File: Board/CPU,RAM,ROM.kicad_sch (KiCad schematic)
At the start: 25 parts, among them IC3 74LVC125, IC6 741G04DBV, IC7 74LVC138, U1 IS61C5128AL-10TLI, X3 SG-8002CE

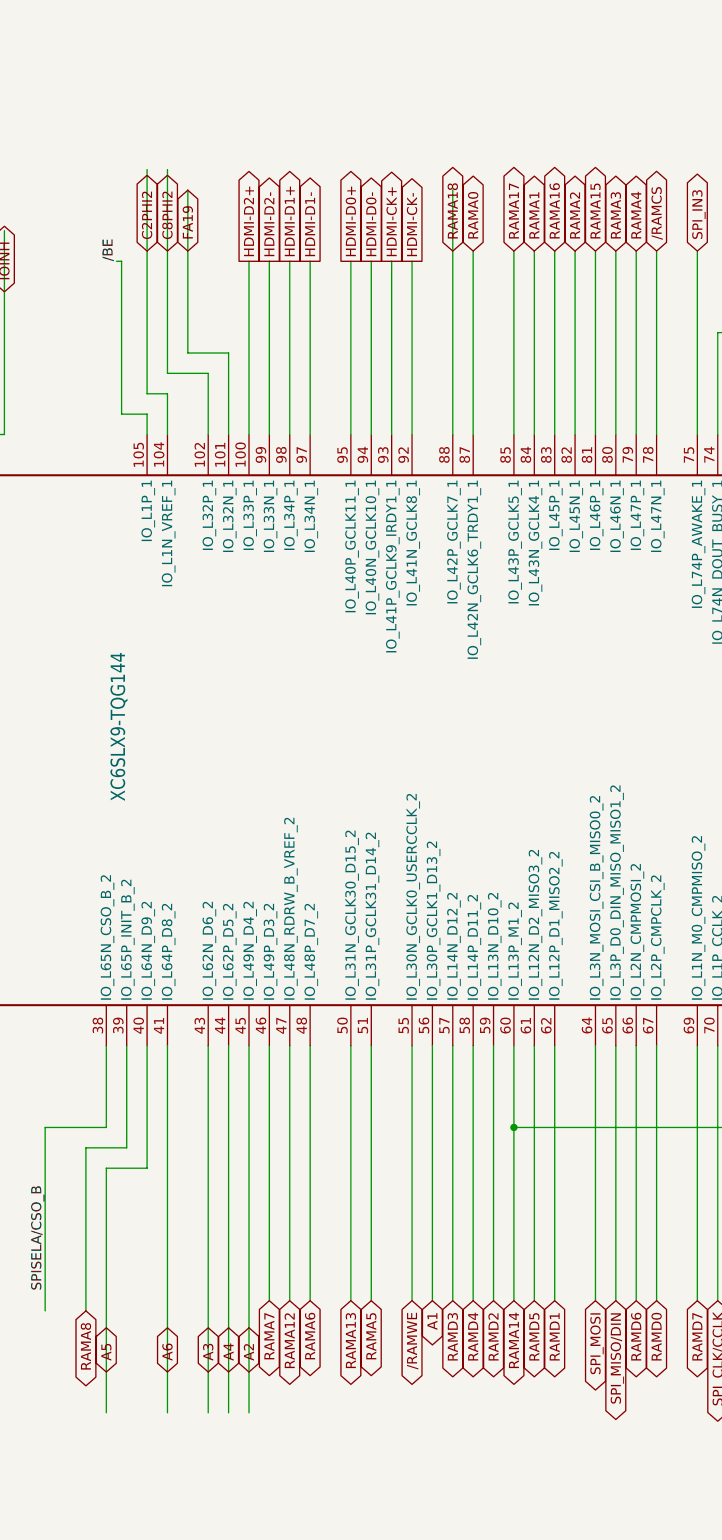
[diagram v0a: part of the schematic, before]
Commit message: update
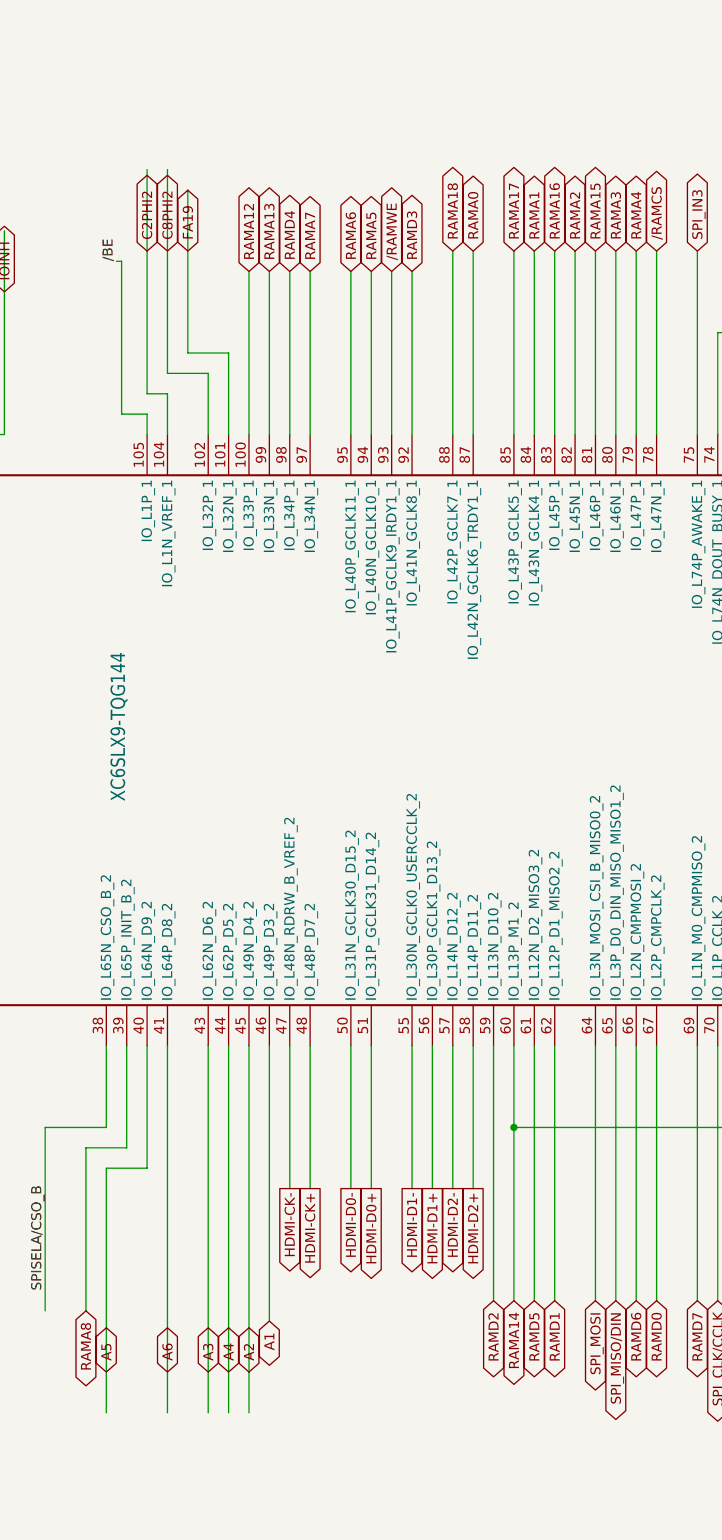
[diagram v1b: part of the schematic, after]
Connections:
- net /RAMWE: now also U$2.93 (IO_L41P_GCLK9_IRDY1_1); no longer U$2.55 (IO_L30N_GCLK0_USERCCLK_2)
- net A1: now also U$2.46 (IO_L49P_D3_2); no longer U$2.56 (IO_L30P_GCLK1_D13_2)
- net HDMI-CK+: now also U$2.48 (IO_L48P_D7_2); no longer U$2.93 (IO_L41P_GCLK9_IRDY1_1)
- net HDMI-CK-: now also U$2.47 (IO_L48N_RDRW_B_VREF_2); no longer U$2.92 (IO_L41N_GCLK8_1)
- net HDMI-D0+: now also U$2.51 (IO_L31P_GCLK31_D14_2); no longer U$2.95 (IO_L40P_GCLK11_1)
- net HDMI-D0-: now also U$2.50 (IO_L31N_GCLK30_D15_2); no longer U$2.94 (IO_L40N_GCLK10_1)
- net HDMI-D1+: now also U$2.56 (IO_L30P_GCLK1_D13_2); no longer U$2.98 (IO_L34P_1)
- net HDMI-D1-: now also U$2.55 (IO_L30N_GCLK0_USERCCLK_2); no longer U$2.97 (IO_L34N_1)
- net HDMI-D2+: now also U$2.58 (IO_L14P_D11_2); no longer U$2.100 (IO_L33P_1)
- net HDMI-D2-: now also U$2.57 (IO_L14N_D12_2); no longer U$2.99 (IO_L33N_1)
- net RAMA12: now also U$2.100 (IO_L33P_1); no longer U$2.47 (IO_L48N_RDRW_B_VREF_2)
- net RAMA13: now also U$2.99 (IO_L33N_1); no longer U$2.50 (IO_L31N_GCLK30_D15_2)
- net RAMA5: now also U$2.94 (IO_L40N_GCLK10_1); no longer U$2.51 (IO_L31P_GCLK31_D14_2)
- net RAMA6: now also U$2.95 (IO_L40P_GCLK11_1); no longer U$2.48 (IO_L48P_D7_2)
- net RAMA7: now also U$2.97 (IO_L34N_1); no longer U$2.46 (IO_L49P_D3_2)
- net RAMD3: now also U$2.92 (IO_L41N_GCLK8_1); no longer U$2.57 (IO_L14N_D12_2)
- net RAMD4: now also U$2.98 (IO_L34P_1); no longer U$2.58 (IO_L14P_D11_2)

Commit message: start working on 3.0 with larger FPGA
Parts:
- removed D9: 1N4448, csa_ultracpu:D-5, symbol csa_ultracpu-eagle-import:DIODE-D-5
- removed unit 2 of IC3
- removed unit 1 of IC3
- removed unit 1 of IC7
- removed JP1, JP4: JP1E, csa_ultracpu:JP1, symbol csa_ultracpu-eagle-import:JP1E
- removed R25, R26: 10k, Resistor_SMD:R_0805_2012Metric_Pad1.20x1.40mm_HandSolder, symbol csa_ultracpu-eagle-import:R-EU_0207/2V
- removed R29: 330, csa_ultracpu:0207_2V, symbol csa_ultracpu-eagle-import:R-EU_0207/2V
- removed U$2: XC6SLX9-TQG144, csa_ultracpu:TQFP144, symbol csa_ultracpu-eagle-import:XC9SLX9-TQG144
- removed unit 2 of U$7
- removed unit 1 of U$7
- removed U1: IS61C5128AL-10TLI, Package_SO:TSOP-II-44_10.16x18.41mm_P0.8mm, symbol Memory_RAM:IS61C5128AL-10TLI
- added U1: IS61WV51216EDALL, Package_SO:TSOP-II-44_10.16x18.41mm_P0.8mm, symbol csa_ultracpu-eagle-import:IS61WV51216EDALL
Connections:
- net A0: now also U1.1 (A0)
- net A1: now also U1.2 (A1)
- net A10: now also U1.23 (A10)
- net A11: now also U1.24 (A11)
- net A2: now also U1.3 (A2)
- net A3: now also U1.4 (A3)
- net A4: now also U1.5 (A4)
- net A5: now also U1.18 (A5)
- net A6: now also U1.19 (A6)
- net A7: now also U1.20 (A7)
- net A8: now also U1.21 (A8)
- net A9: now also U1.22 (A9)
- net D0: now also U1.29 (I/O8), U1.7 (I/O0)
- net D1: now also U1.30 (I/O9), U1.8 (I/O1)
- net D2: now also U1.31 (I/O10), U1.9 (I/O2)
- net D3: now also U1.10 (I/O3), U1.32 (I/O11)
- net D4: now also U1.13 (I/O4), U1.35 (I/O12)
- net D5: now also U1.14 (I/O5), U1.36 (I/O13)
- net D6: now also U1.15 (I/O6), U1.37 (I/O14)
- net D7: now also U1.16 (I/O7), U1.38 (I/O15)
- net FA15: now also U1.42 (A15)
- net FA16: now also U1.43 (A16)
- net FA17: now also U1.44 (A17)
- net FA18: now also U1.28 (A18)
- net GND: now also U1.12 (GND), U1.34 (GND)
- net R/-W: now also U1.17 (~{WE})
- net V33: now also U1.11 (VDD), U1.33 (VDD)
- net /FRAMSEL: now also U1.41 (~{OE}), U1.6 (~{CE})
- net 50M renamed QCLK
- new net FA12: U1.25 (A12)
- new net FA13: U1.26 (A13)
- new net FA14: U1.27 (A14)
- new net /FRAMLB: U1.39 (~{LB})
- new net /FRAMUB: U1.40 (~{UB})
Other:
- note added: "CSA-UTRACPU-V3.0A"
- note added: "Fast RAM"
- note added: "V2.0A: - use CCLK for all SPI clocks - add switchable CPU BE input - VCCAUX is 3.3V now - Added test points V2.0B: - IC6 power supply to 3.3V instead of 5V - Pulldown /RES as long as DONE is low V2.1A: - use TSOP-II 44 pin package for SRAM - use 3225 package for 54MHz SMD oscillator V3.0A: - go from VGA to HDMI - go to larger FPGA in BGA package, move FPGA to own page - use 16bit Fast RAM IC"
- note removed: "CSA-UTRACPU-V2.2A"
- note removed: "For Master SPI config, M[0..1] need to be 01 (M0=1, M1=0) - doing this with '125 when DONE is low M[] are sampled when INIT_B goes high, std I/O after config DONE goes high after initialization is finished. Boot PROM connections: MOSI is SPI MOSI DIN is SPI MISO CSO_B is Boot flash /select CCLK is SPI clock (CCLK is 50 Ohm transmission line - no branches 100/100 termination)"
- note removed: "HSWAP pulldown during configuration to enable pullups on config+I/O pins"
- note removed: "Protection against accidently connecting the wrong way around"
- note removed: "Pulling M1 to low for SPI master config on FPGA boot"
- note removed: "V2.0A: - use CCLK for all SPI clocks - add switchable CPU BE input - VCCAUX is 3.3V now - Added test points V2.0B: - IC6 power supply to 3.3V instead of 5V - Pulldown /RES as long as DONE is low V2.1A: - use TSOP-II 44 pin package for SRAM - use 3225 package for 54MHz SMD oscillator V2.2A: - go from VGA to HDMI"
- moved on the sheet: IC3C, IC3E, IC6A, IC6B, IC7B, JP10, JP11, JP7, JP8, JP9, R10, R11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
